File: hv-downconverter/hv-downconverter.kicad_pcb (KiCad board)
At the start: 2 copper layers, 95 x 62 mm, 24 parts, among them J1 Conn_01x02_Pin, J2 Conn_01x02_Pin, Q1 Q_NMOS_GDS, Q2 Q_NMOS_GDS, U1 LM5116MHX/NOPB

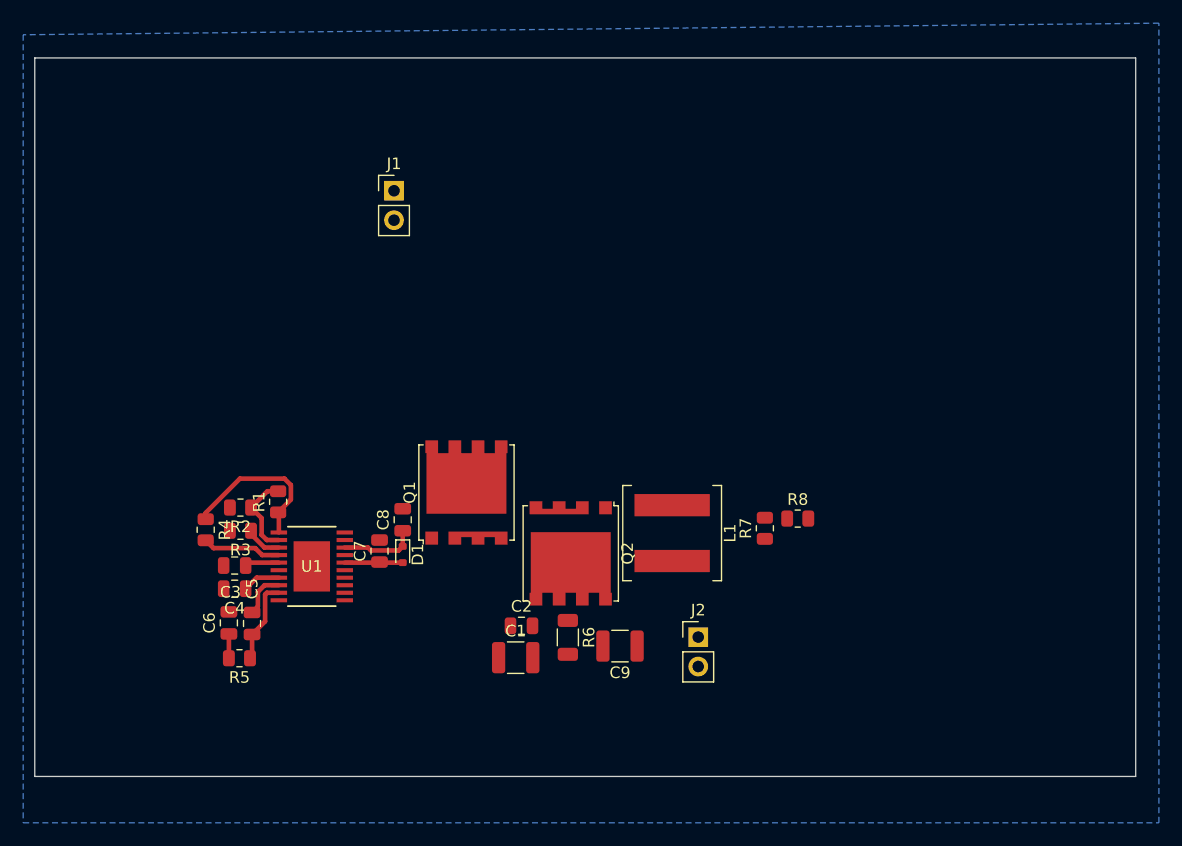
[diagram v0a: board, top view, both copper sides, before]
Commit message: almost ready for fab
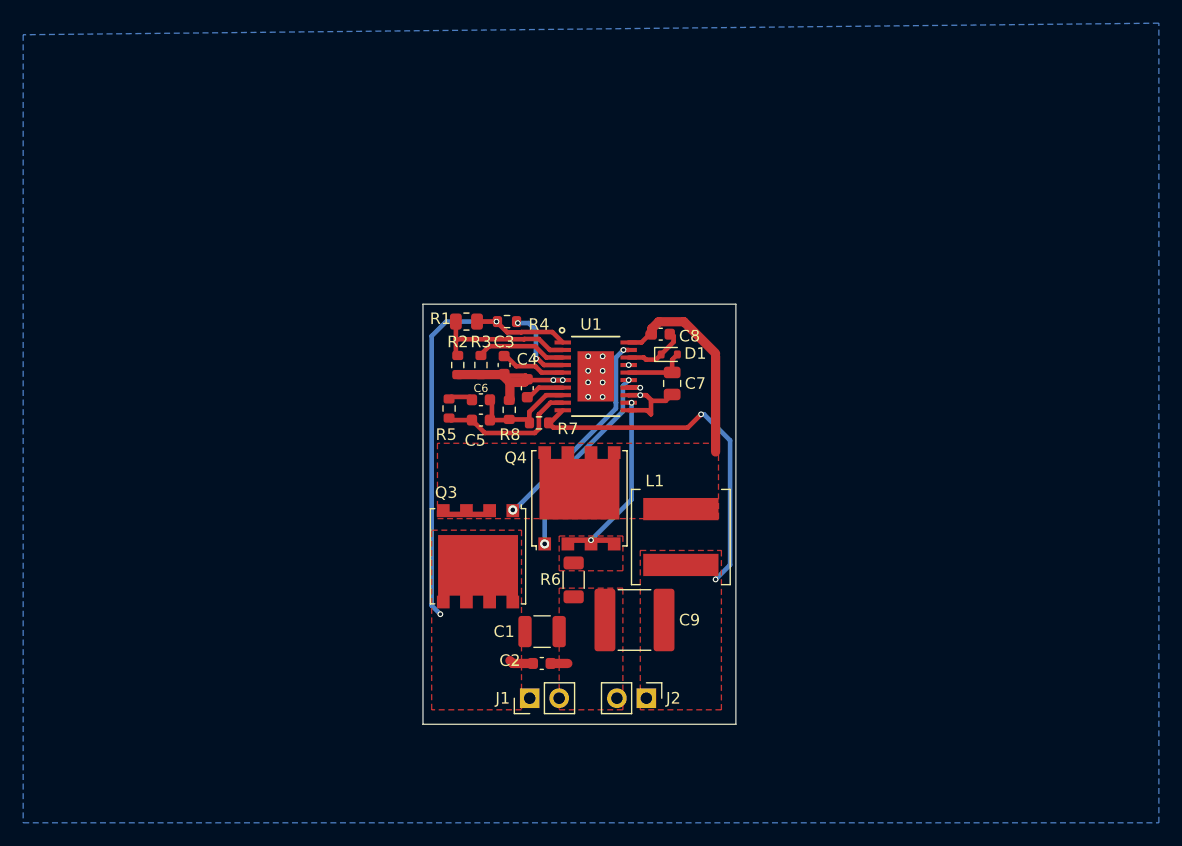
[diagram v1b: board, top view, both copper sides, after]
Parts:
- removed Q1, Q2: Q_NMOS_GDS, Package_TO_SOT_SMD:PQFN_8x8
- added Q3: Q_NMOS_GSD, Package_TO_SOT_SMD:PQFN_8x8, F.Cu at (167.2, 87.0)
- added Q4: Q_NMOS_GSD, Package_TO_SOT_SMD:PQFN_8x8, F.Cu at (176.0, 82.0)
- C2, C3, C4, C5, C6, C8: footprint Capacitor_SMD:C_0805_2012Metric -> Capacitor_SMD:C_0603_1608Metric
- C9: footprint Capacitor_SMD:C_1210_3225Metric -> Capacitor_SMD:C_2220_5650Metric
- R2, R3, R4, R5, R7, R8: footprint Resistor_SMD:R_0805_2012Metric -> Resistor_SMD:R_0603_1608Metric
- moved J1 45.3 mm to (171.7, 99.2), turned to 90 degrees
- moved R4 31.6 mm to (169.8, 66.8), turned to 0 degrees
- moved C4 30.6 mm to (171.5, 72.5), turned to 90 degrees
- moved U1 29.5 mm to (177.4, 71.5)
- moved C7 29.1 mm to (184.0, 72.1), turned to -90 degrees
- moved C6 29.0 mm to (167.5, 73.5), turned to 0 degrees
- moved C3 29.0 mm to (169.5, 70.5), turned to -90 degrees
- moved D1 28.8 mm to (183.8, 69.6), turned to 0 degrees
- moved R5 28.1 mm to (164.8, 74.2), turned to 90 degrees
- moved C8 27.4 mm to (183.0, 67.8), turned to 180 degrees
- moved R8 26.6 mm to (169.9, 74.4), turned to 90 degrees
- moved C5 26.4 mm to (167.5, 75.2), turned to 0 degrees
- moved R3 25.2 mm to (167.5, 70.5), turned to -90 degrees
- moved R1 22.5 mm to (166.2, 66.8), turned to 180 degrees
- moved R2 22.4 mm to (165.5, 70.5), turned to -90 degrees
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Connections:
- U1 pad 21: unconnected-(U1-DAP-Pad21) -> GND
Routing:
- net Net-(J2-Pin_1): track 0.00 -> 31.5 mm, vias 0 -> 2
- net GND: track 0.00 -> 29.2 mm, vias 0 -> 13
- net Net-(J1-Pin_1): track 14.0 -> 40.7 mm, vias 0 -> 2
- net Net-(Q3-G): track 0.00 -> 18.3 mm, vias 0 -> 2
- net Net-(Q3-S): track 0.00 -> 17.8 mm
- net Net-(Q4-G): track 0.00 -> 17.2 mm, vias 0 -> 2
- net Net-(Q4-S): track 0.00 -> 13.3 mm, vias 0 -> 2
- net Net-(U1-FB): track 4.03 -> 9.95 mm
- net Net-(U1-UVLO): track 7.32 -> 12.5 mm
- net Net-(U1-COMP): track 7.29 -> 12.0 mm
- net Net-(U1-RT/SYNC): track 3.17 -> 7.76 mm
- net Net-(U1-RAMP): track 2.96 -> 5.72 mm
- net Net-(D1-K): track 6.60 -> 5.32 mm
- net Net-(U1-EN): track 6.84 -> 6.95 mm, vias 0 -> 2
- added copper zone on F.Cu, net GND
- added copper zone on In1.Cu, net GND
- added copper zone on In2.Cu, net GND
- added copper zone on F.Cu, net Net-(J1-Pin_1)
- added copper zone on F.Cu, net Net-(J2-Pin_1)
- added copper zone on F.Cu, net Net-(Q3-S)
- added copper zone on F.Cu, net Net-(Q4-S)
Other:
- board size 95 x 62 mm -> 27 x 36.2 mm
- copper layers 2 -> 4
